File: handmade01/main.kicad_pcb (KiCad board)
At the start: 2 copper layers, 64.8 x 70.1 mm, 71 parts, among them CON1 MicroSD, CON2 MicroSD, J1 JACK_TRS_6PINS, P1 VOLUMN, P4 USB_OTG, P6 UART_DEBUG, Q1 1AM, SW1 Power, SW10 R, SW11 A, SW12 B, SW13 X, SW14 Y, SW2 Reset, SW3 UP, SW4 Down, SW5 Left, SW6 Right, SW7 Select, SW8 Start, SW9 L, U1 PCM5102A, U2 PAM8403, U3 IPS_2.4_240x320_ST7789V, U4 CM3354, U5 TPS71718

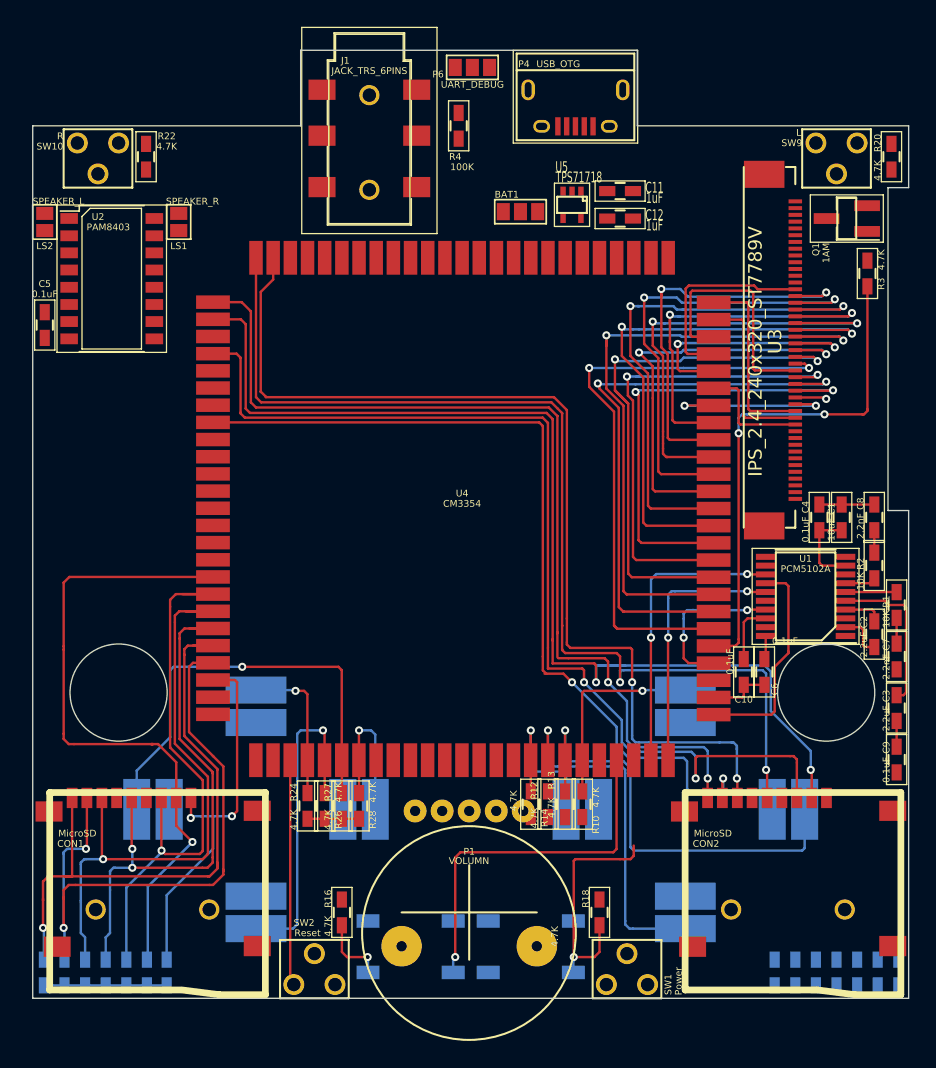
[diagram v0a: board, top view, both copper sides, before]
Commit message: 20171215
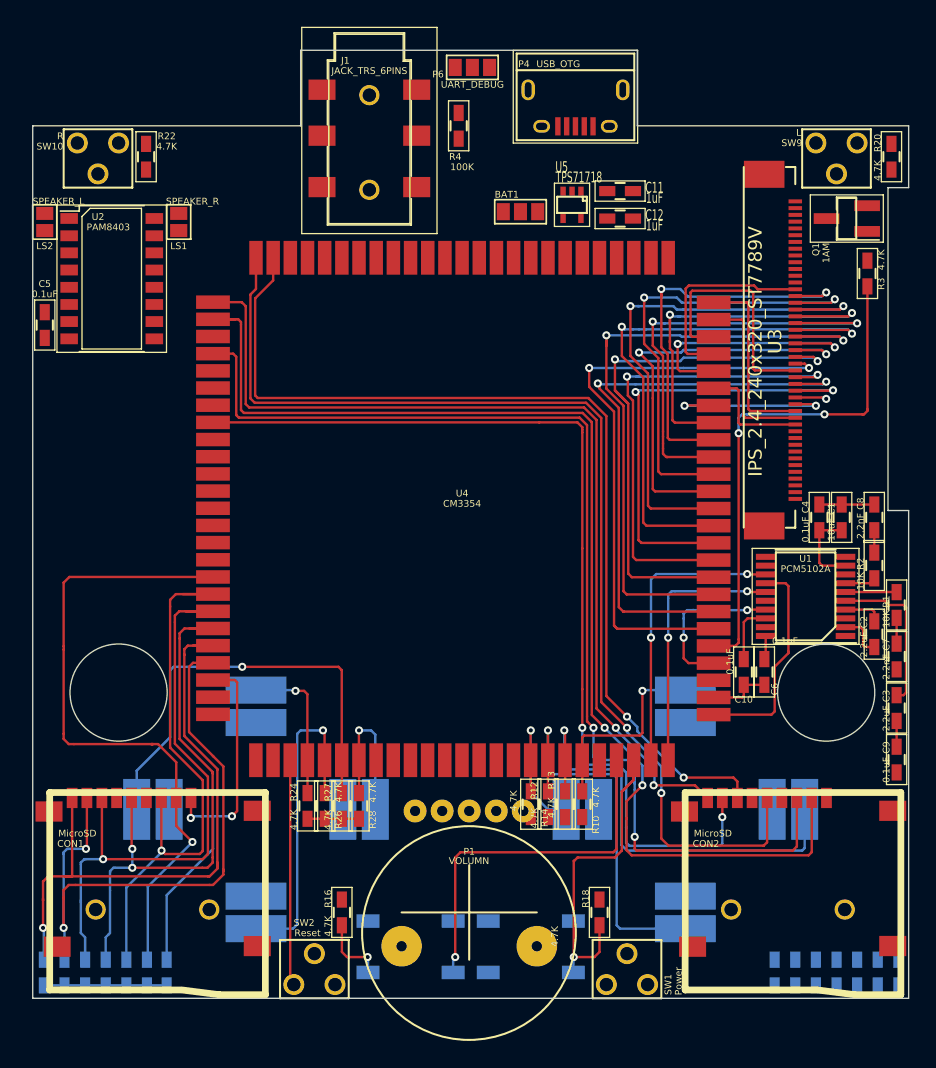
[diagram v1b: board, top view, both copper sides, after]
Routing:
- net START: track 18.1 -> 26.3 mm
- net SD1_DAT3: track 64.2 -> 71.6 mm
- net SD1_DAT1: track 81.6 -> 88.4 mm
- net SD1_DAT0: track 76.3 -> 82.9 mm
- net SD1_CLK: track 78.5 -> 81.5 mm
- net SD1_CMD: track 74.4 -> 71.7 mm
- net DOWN: track 26.7 -> 28.9 mm
- net SD1_DAT2: track 70.8 -> 69.5 mm
